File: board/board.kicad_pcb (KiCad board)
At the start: 4 copper layers, 53 x 39.5 mm, 36 parts, among them J1 ANT, J2 DEBUG, J3 GPIO, P1 USB_C_Plug_USB2.0, SW1 BOOTSEL, SW2 RUN, U1 RP2040, U2 W25Q128JVS, U3 NCP1117-3.3_SOT223, U4 RFM95W-915S2, U5 BLE5201, Y1 ABM8G-12.000MHZ-18-D2Y-T

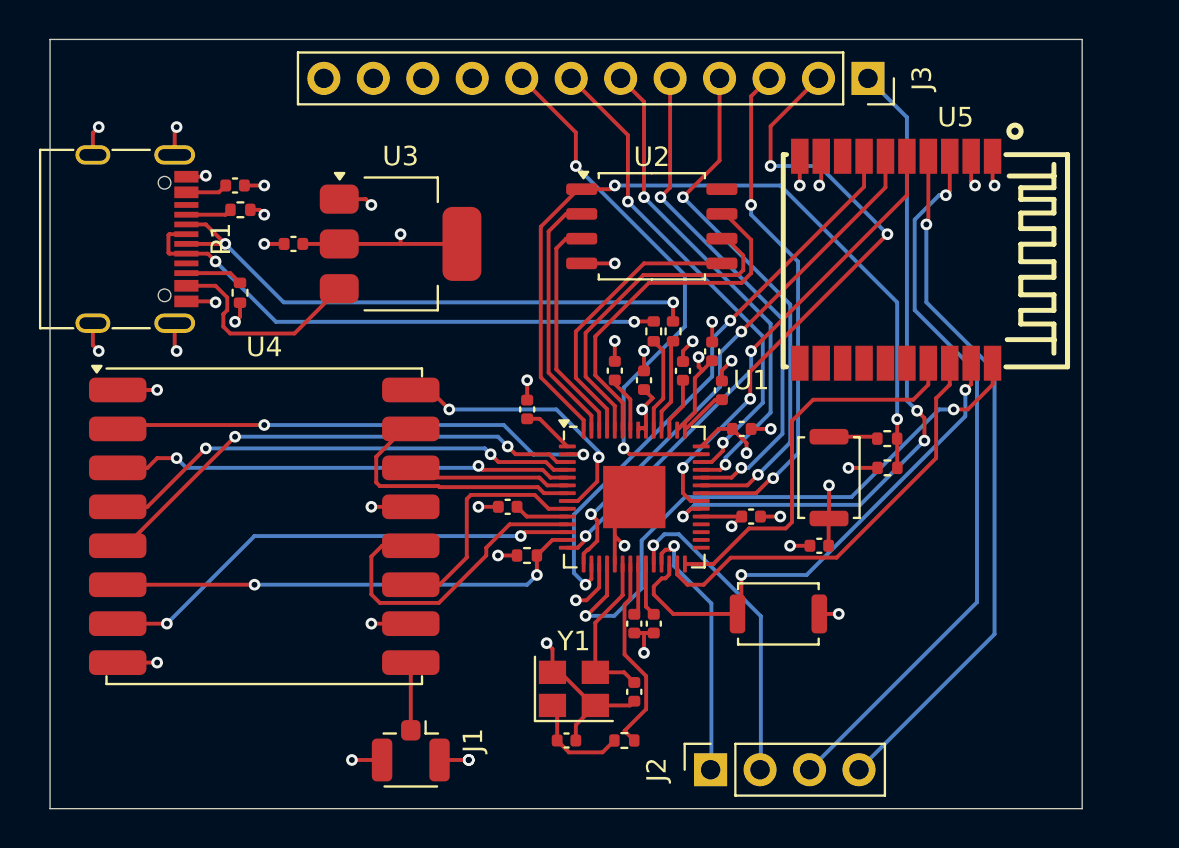
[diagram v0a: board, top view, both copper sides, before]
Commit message: finish board v2
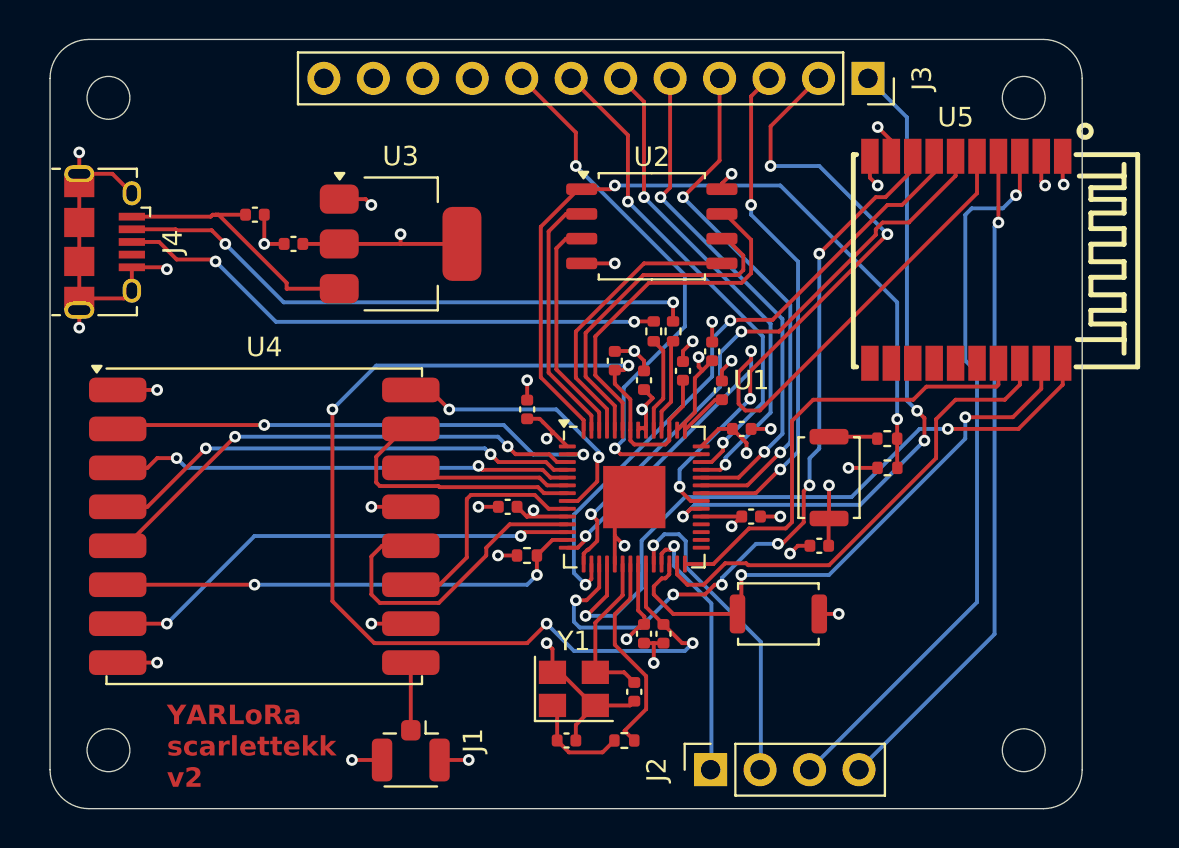
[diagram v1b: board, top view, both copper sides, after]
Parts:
- removed P1: USB_C_Plug_USB2.0, Connector_USB:USB_C_Receptacle_G-Switch_GT-USB-7010ASV
- removed R3, R4: 5.1k, Resistor_SMD:R_0402_1005Metric
- added J4: USB_B_Micro, Connector_USB:USB_Micro-B_Amphenol_10118194_Horizontal, F.Cu at (44.8, 36.9)
- added REF**: MountingHole_2.2mm_M2, MountingHole:MountingHole_2.2mm_M2, F.Cu at (45.0, 29.5)
- added REF**: MountingHole_2.2mm_M2, MountingHole:MountingHole_2.2mm_M2, F.Cu at (92.0, 29.5)
- added REF**: MountingHole_2.2mm_M2, MountingHole:MountingHole_2.2mm_M2, F.Cu at (45.0, 63.0)
- added REF**: MountingHole_2.2mm_M2, MountingHole:MountingHole_2.2mm_M2, F.Cu at (92.0, 63.0)
- moved U5 3.60 mm to (89.0, 37.8)
- moved C12 1.81 mm to (52.5, 35.5)
- moved C3 0.72 mm to (72.5, 57.0)
- moved C9 0.72 mm to (73.5, 57.0)
- moved C10 0.51 mm to (71.0, 43.0)
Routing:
- net +1V1: track 8.50 -> 62.2 mm, vias 0 -> 4
- net Net-(U1-GPIO14): track 2.68 -> 39.6 mm, vias 1 -> 6
- net Net-(U1-GPIO11): track 27.6 -> 36.2 mm
- net GND: track 57.3 -> 64.5 mm, vias 34 -> 26
- net +3V3: track 42.4 -> 46.7 mm, vias 11 -> 15
- net /PB02: track 20.6 -> 24.2 mm
- net /PB00: track 31.5 -> 35.1 mm
- net /RUN: track 26.5 -> 30.1 mm
- net Net-(U1-GPIO12): track 27.7 -> 31.1 mm
- net Net-(U1-GPIO13): track 29.6 -> 32.8 mm
- net /PB01: track 21.9 -> 25.0 mm
- net Net-(P1-CC2): track 2.96 -> 0.00 mm
- net Net-(P1-CC1): track 2.37 -> 0.00 mm
- net /BLE_SWDIO: track 35.9 -> 34.5 mm
- net VBUS: track 13.1 -> 14.0 mm
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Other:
- outline, holes or cut-outs redrawn
- board text added: "YARLoRa scarlettekk v2"
